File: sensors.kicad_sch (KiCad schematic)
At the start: 43 parts

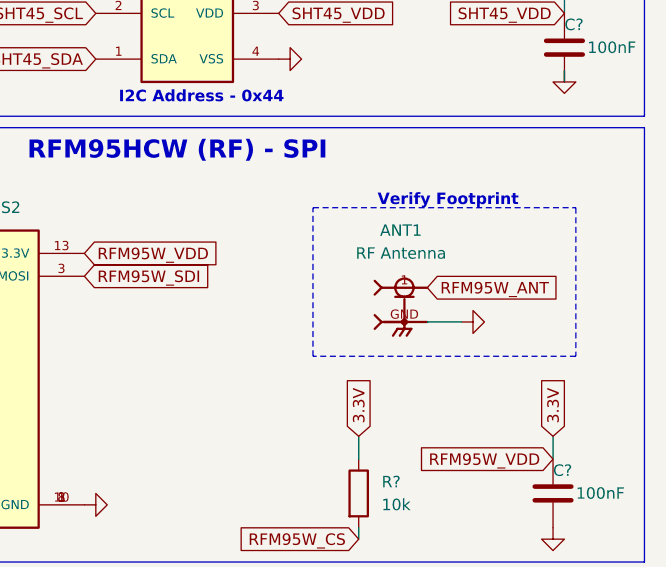
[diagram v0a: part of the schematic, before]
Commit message: updated pcb
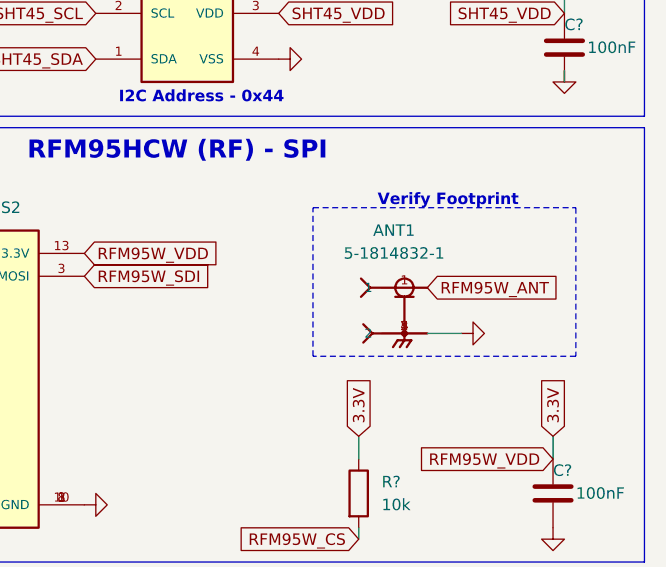
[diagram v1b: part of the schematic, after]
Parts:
- removed ANT1: RF Antenna, 5449692-1:TE_5449692-1, symbol 5449692-1:5449692-1
- added ANT1: 5-1814832-1, 5-1814832-1:TE_5-1814832-1, symbol 5-1814832-1:5-1814832-1
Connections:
- net GND: now also ANT1.2, ANT1.3 (2), ANT1.4 (2), ANT1.5 (2)
- net RFM95W_ANT: now also ANT1.1
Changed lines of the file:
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@@
     (stroke (width 0) (type default))
   )
-  (wire (pts (xy 264.16 137.16) (xy 260.35 137.16))
+  (wire (pts (xy 264.16 138.43) (xy 260.35 138.43))
     (stroke (width 0) (type default))
   )
@@
     )
   )
-  (symbol (lib_id "power:GND") (at 264.16 137.16 90) (unit 1)
-    (in_bom yes) (on_board yes) (dnp no) (fields_autoplaced)
-    (property "Reference" "#PWR?" (at 270.51 137.16 0)
-      (effects (font (size 1.27 1.27)) hide)
-    )
-    (property "Value" "GND" (at 267.97 137.16 90)
-      (effects (font (size 1.27 1.27)) (justify right) hide)
-    )
-    (property "Footprint" "" (at 264.16 137.16 0)
-      (effects (font (size 1.27 1.27)) hide)
-    )
-    (property "Datasheet" "" (at 264.16 137.16 0)
+  (symbol (lib_id "power:GND") (at 264.16 138.43 90) (unit 1)
+    (in_bom yes) (on_board yes) (dnp no) (fields_autoplaced)
+    (property "Reference" "#PWR?" (at 270.51 138.43 0)
+      (effects (font (size 1.27 1.27)) hide)
+    )
+    (property "Value" "GND" (at 267.97 138.43 90)
+      (effects (font (size 1.27 1.27)) (justify right) hide)
+    )
+    (property "Footprint" "" (at 264.16 138.43 0)
+      (effects (font (size 1.27 1.27)) hide)
+    )
+    (property "Datasheet" "" (at 264.16 138.43 0)
       (effects (font (size 1.27 1.27)) hide)
     )
@@
         (path "/e12346fa-509d-4de9-8ab1-dced307292db/b5ec7ecd-943d-4169-981a-c46b6432f873"
           (reference "R30") (unit 1)
-        )
-      )
-    )
-  )
-  (symbol (lib_id "5449692-1:5449692-1") (at 257.81 137.16 0) (unit 1)
-    (in_bom yes) (on_board yes) (dnp no) (fields_autoplaced)
-    (property "Reference" "ANT1" (at 257.429 127 0)
-      (effects (font (size 1.27 1.27)))
-    )
-    (property "Value" "RF Antenna" (at 257.429 129.54 0)
-      (effects (font (size 1.27 1.27)))
-    )
-    (property "Footprint" "5449692-1:TE_5449692-1" (at 257.81 142.24 0)
-      (effects (font (size 1.27 1.27)) (justify bottom) hide)
-    )
-    (property "Datasheet" "" (at 257.81 137.16 0)
-      (effects (font (size 1.27 1.27)) hide)
-    )
-    (property "Comment" "5449692-1" (at 257.81 140.97 0)
-      (effects (font (size 1.27 1.27)) (justify bottom) hide)
-    )
-    (pin "1")
-    (pin "GND")
-    (pin "GND")
-    (instances
-      (project "aether"
-        (path "/e12346fa-509d-4de9-8ab1-dced307292db/b5ec7ecd-943d-4169-981a-c46b6432f873"
-          (reference "ANT1") (unit 1)
         )
       )
@@
         )
       )
+    )
+  )
+  (symbol (lib_id "5-1814832-1:5-1814832-1") (at 257.81 135.89 0) (unit 1)
+    (in_bom yes) (on_board yes) (dnp no) (fields_autoplaced)
+    (property "Reference" "ANT1" (at 256.667 127 0)
+      (effects (font (size 1.27 1.27)))
+    )
+    (property "Value" "5-1814832-1" (at 256.667 129.54 0)
+      (effects (font (size 1.27 1.27)))
+    )
+    (property "Footprint" "5-1814832-1:TE_5-1814832-1" (at 257.81 135.89 0)
+      (effects (font (size 1.27 1.27)) (justify bottom) hide)
+    )
+    (property "Datasheet" "" (at 257.81 135.89 0)
+      (effects (font (size 1.27 1.27)) hide)
+    )
+    (property "Comment" "5-1814832-1" (at 257.81 135.89 0)
+      (effects (font (size 1.27 1.27)) (justify bottom) hide)
+    )
+    (property "MF" "TE Connectivity" (at 257.81 135.89 0)
+      (effects (font (size 1.27 1.27)) (justify bottom) hide)
+    )
+    (property "Description" "\nConnector SMA JACK STR 50 OHM PCB | TE Connectivity 5-1814832-1\n" (at 257.81 135.89 0)
+      (effects (font (size 1.27 1.27)) (justify bottom) hide)
+    )
+    (property "Package" "None" (at 257.81 135.89 0)
+      (effects (font (size 1.27 1.27)) (justify bottom) hide)
+    )
+    (property "Price" "None" (at 257.81 135.89 0)
+      (effects (font (size 1.27 1.27)) (justify bottom) hide)
+    )
+    (property "Check_prices" "https://www.snapeda.com/parts/5-1814832-1/TE+Connectivity+AMP+Connectors/view-part/?ref=eda" (at 257.81 135.89 0)
+      (effects (font (size 1.27 1.27)) (justify bottom) hide)
+    )
+    (property "STANDARD" "Manufacturer recommendations" (at 257.81 135.89 0)
+      (effects (font (size 1.27 1.27)) (justify bottom) hide)
+    )
+    (property "PARTREV" "B1" (at 257.81 135.89 0)
+      (effects (font (size 1.27 1.27)) (justify bottom) hide)
+    )
+    (property "SnapEDA_Link" "https://www.snapeda.com/parts/5-1814832-1/TE+Connectivity+AMP+Connectors/view-part/?ref=snap" (at 257.81 135.89 0)
+      (effects (font (size 1.27 1.27)) (justify bottom) hide)
+    )
+    (property "MP" "5-1814832-1" (at 257.81 135.89 0)
+      (effects (font (size 1.27 1.27)) (justify bottom) hide)
+    )
+    (property "Purchase-URL" "https://www.snapeda.com/api/url_track_click_mouser/?unipart_id=38815&manufacturer=TE Connectivity&part_name=5-1814832-1&search_term=5-1814832-1" (at 257.81 135.89 0)
+      (effects (font (size 1.27 1.27)) (justify bottom) hide)
+    )
+    (property "EU_RoHS_Compliance" "Compliant with Exemptions" (at 257.81 135.89 0)
+      (effects (font (size 1.27 1.27)) (justify bottom) hide)
+    )
+    (property "Number_of_Positions" "1" (at 257.81 135.89 0)
+      (effects (font (size 1.27 1.27)) (justify bottom) hide)
+    )
+    (property "Availability" "In Stock" (at 257.81 135.89 0)
+      (effects (font (size 1.27 1.27)) (justify bottom) hide)
+    )
+    (property "MANUFACTURER" "TE Connectivity" (at 257.81 135.89 0)
+      (effects (font (size 1.27 1.27)) (justify bottom) hide)
+    )
+    (pin "1")
+    (pin "2")
+    (pin "3")
+    (pin "4")
+    (pin "5")
+    (instances
+      (project "aether"
+        (path "/e12346fa-509d-4de9-8ab1-dced307292db/b5ec7ecd-943d-4169-981a-c46b6432f873"
+          (reference "ANT1") (unit 1)
+        )
+      )
